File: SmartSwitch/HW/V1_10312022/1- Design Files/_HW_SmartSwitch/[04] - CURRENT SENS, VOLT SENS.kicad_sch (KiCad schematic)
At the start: 0 parts

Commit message: Current sensor has been done almost :D
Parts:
- added C?: 100nF/16V, Capacitor_SMD:C_0402_1005Metric, symbol SmartSwitch:100nF/16V
- added C?: 1uF/16V, Capacitor_SMD:C_0402_1005Metric, symbol SmartSwitch:1uF/16V
- added C? (x2): 4n7F/25V, Capacitor_SMD:C_0402_1005Metric, symbol SmartSwitch:4n7F/25V
- added D? (x2): PESD3V3X1BCSFYL, symbol SmartSwitch:PESD3V3X1BCSFYL
- added R?: 1MR_1/20W, Resistor_SMD:R_0201_0603Metric, symbol SmartSwitch:1MR_1/20W
- added R? (x2): 470KR_1/16W, Resistor_SMD:R_0402_1005Metric, symbol SmartSwitch:470KR_1/16W
- added R?: 0.01R_10W, Resistor_SMD:R_2816_7142Metric_Pad3.20x4.45mm_HandSolder, symbol SmartSwitch:0.01R_10W
- added R? (x2): 33KR_1/16W, Resistor_SMD:R_0402_1005Metric, symbol SmartSwitch:33KR_1/16W
- added R?: 100R_1/20W, Resistor_SMD:R_0201_0603Metric, symbol SmartSwitch:100R_1/20W
- added U?: MCP6006UT, Package_TO_SOT_SMD:SOT-23-5, symbol SmartSwitch:MCP6006UT
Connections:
- new net: C?.2, D?.1, R?.2, R?.2, U?.1 (VIN+)
- new net: C?.1, D?.1, R?.1, R?.2, U?.3 (VIN-)
- new net: C?.2, R?.1, R?.2, U?.4 (VOUT)
- new net +3V3: C?.2, C?.2, U?.5 (VDD)
- new net ADC_CURRENT: R?.2, R?.2
- new net GND: C?.1, C?.1, C?.1, D?.2, D?.2, R?.1, R?.1, U?.2 (VSS)
- new net HOT_Line: R?.1, R?.2
- new net LOAD: R?.1, R?.1

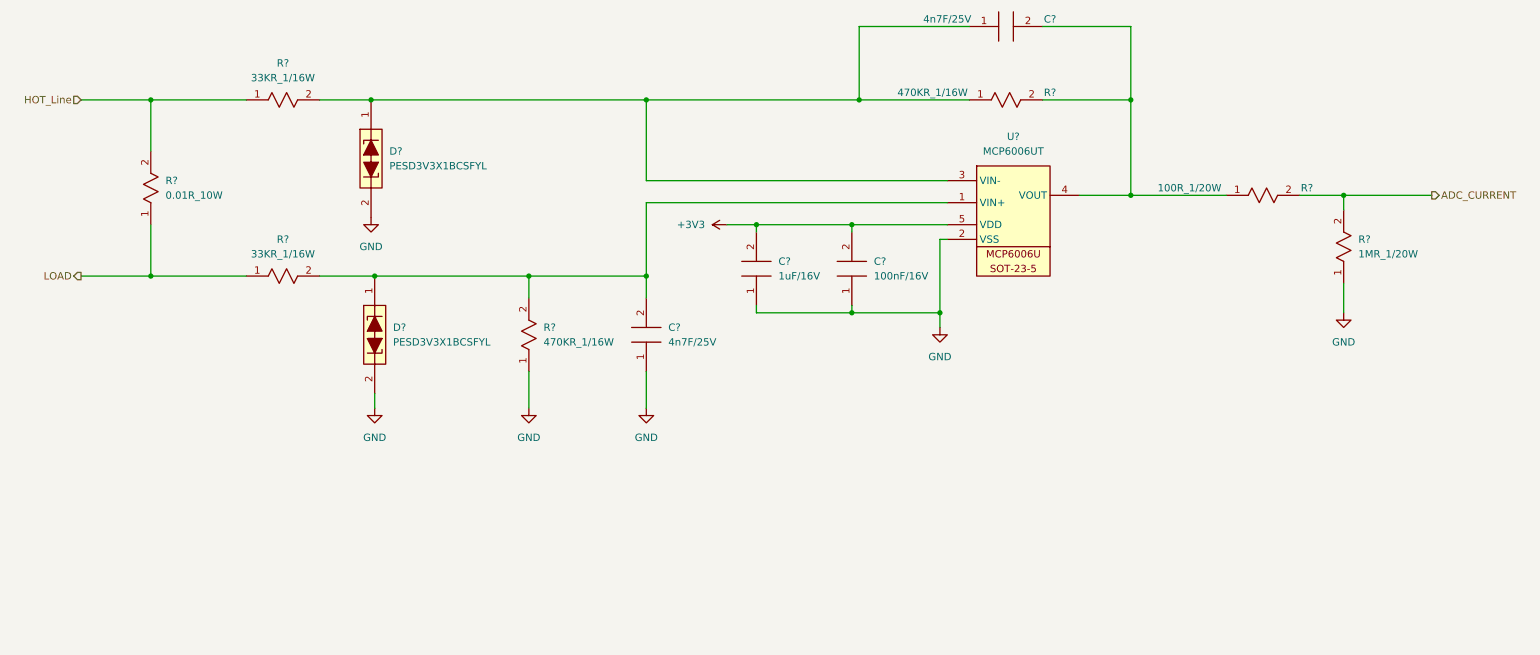
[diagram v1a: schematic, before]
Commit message: Current and Voltage sampler
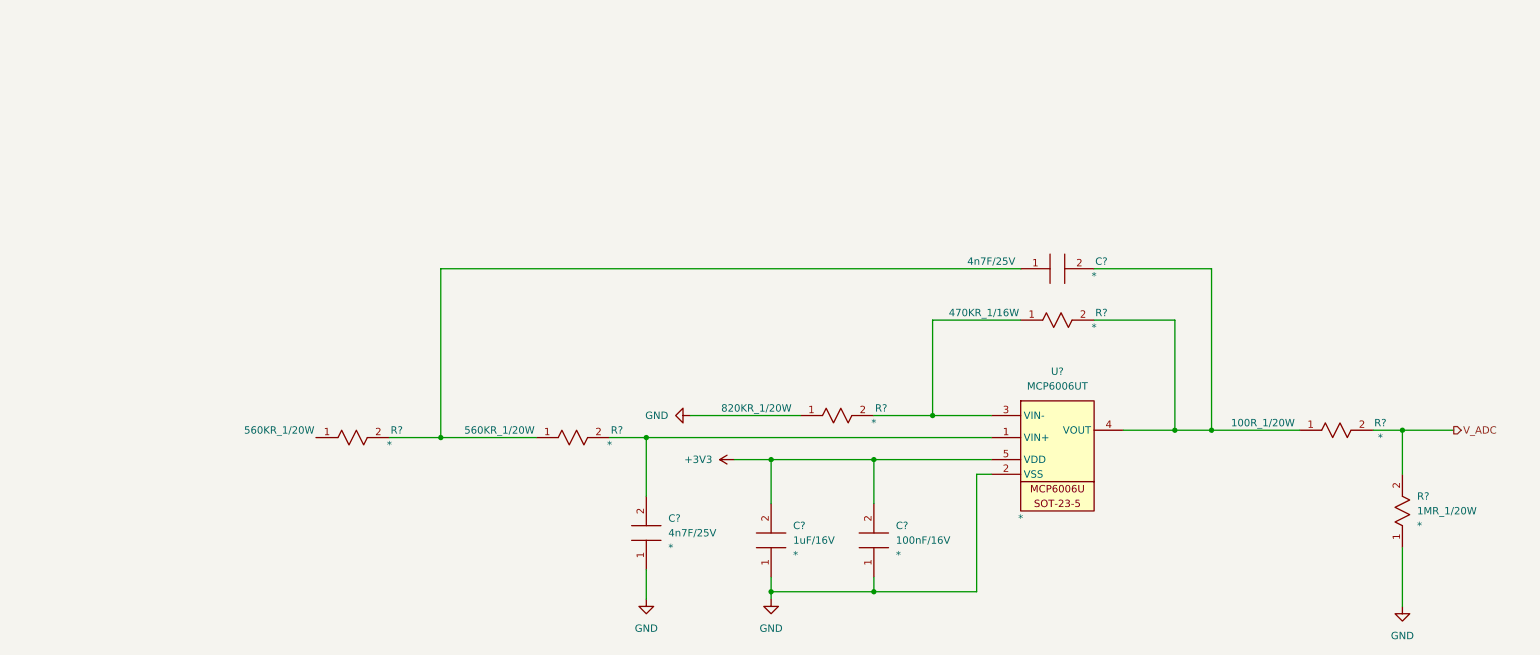
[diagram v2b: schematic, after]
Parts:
- removed C?: 100nF/16V, Capacitor_SMD:C_0402_1005Metric, symbol SmartSwitch:100nF/16V
- removed C?: 1uF/16V, Capacitor_SMD:C_0402_1005Metric, symbol SmartSwitch:1uF/16V
- removed C? (x2): 4n7F/25V, Capacitor_SMD:C_0402_1005Metric, symbol SmartSwitch:4n7F/25V
- removed D? (x2): PESD3V3X1BCSFYL, symbol SmartSwitch:PESD3V3X1BCSFYL
- removed R?: 1MR_1/20W, Resistor_SMD:R_0201_0603Metric, symbol SmartSwitch:1MR_1/20W
- removed R? (x2): 470KR_1/16W, Resistor_SMD:R_0402_1005Metric, symbol SmartSwitch:470KR_1/16W
- removed R?: 0.01R_10W, Resistor_SMD:R_2816_7142Metric_Pad3.20x4.45mm_HandSolder, symbol SmartSwitch:0.01R_10W
- removed R? (x2): 33KR_1/16W, Resistor_SMD:R_0402_1005Metric, symbol SmartSwitch:33KR_1/16W
- removed R?: 100R_1/20W, Resistor_SMD:R_0201_0603Metric, symbol SmartSwitch:100R_1/20W
- removed U?: MCP6006UT, Package_TO_SOT_SMD:SOT-23-5, symbol SmartSwitch:MCP6006UT
- added C? (x2): 4n7F/25V, Capacitor_SMD:C_0402_1005Metric, symbol SmartSwitch:4n7F/25V
- added C?: 1uF/16V, Capacitor_SMD:C_0402_1005Metric, symbol SmartSwitch:1uF/16V
- added C?: 100nF/16V, Capacitor_SMD:C_0402_1005Metric, symbol SmartSwitch:100nF/16V
- added R? (x2): 560KR_1/20W, Resistor_SMD:R_0201_0603Metric, symbol SmartSwitch:560KR_1/20W
- added R?: 100R_1/20W, Resistor_SMD:R_0201_0603Metric, symbol SmartSwitch:100R_1/20W
- added R?: 1MR_1/20W, Resistor_SMD:R_0201_0603Metric, symbol SmartSwitch:1MR_1/20W
- added R?: 470KR_1/16W, Resistor_SMD:R_0402_1005Metric, symbol SmartSwitch:470KR_1/16W
- added R?: 820KR_1/20W, Resistor_SMD:R_0201_0603Metric, symbol SmartSwitch:820KR_1/20W
- added U?: MCP6006UT, Package_TO_SOT_SMD:SOT-23-5, symbol SmartSwitch:MCP6006UT
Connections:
- net +3V3: now also C?.2, C?.2, U?.5 (VDD)
- net GND: now also C?.1, C?.1, C?.1, R?.1, R?.1, U?.2 (VSS)
- new net: C?.1, R?.1, R?.2
- new net: C?.2, R?.1, R?.2, U?.4 (VOUT)
- new net: C?.2, R?.2, U?.1 (VIN+)
- new net: R?.1, R?.2, U?.3 (VIN-)
- new net V_ADC: R?.2, R?.2
